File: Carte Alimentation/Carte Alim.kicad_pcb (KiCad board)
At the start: 2 copper layers, 102.9 x 70.5 mm, 58 parts, among them K1 CONN_3, P1 CONN_2, P10 CONN_2, P11 CONN_2, P12 CONN_2, P13 CONN_4, P2 CONN_2, P3 CONN_2, P4 CONN_5, P5 CONN_1, P6 CONN_1, P7 CONN_1, P8 CONN_1, P9 CONN_2, U100 7905_CORRIGE, U3 LM2903, U4 LM2903

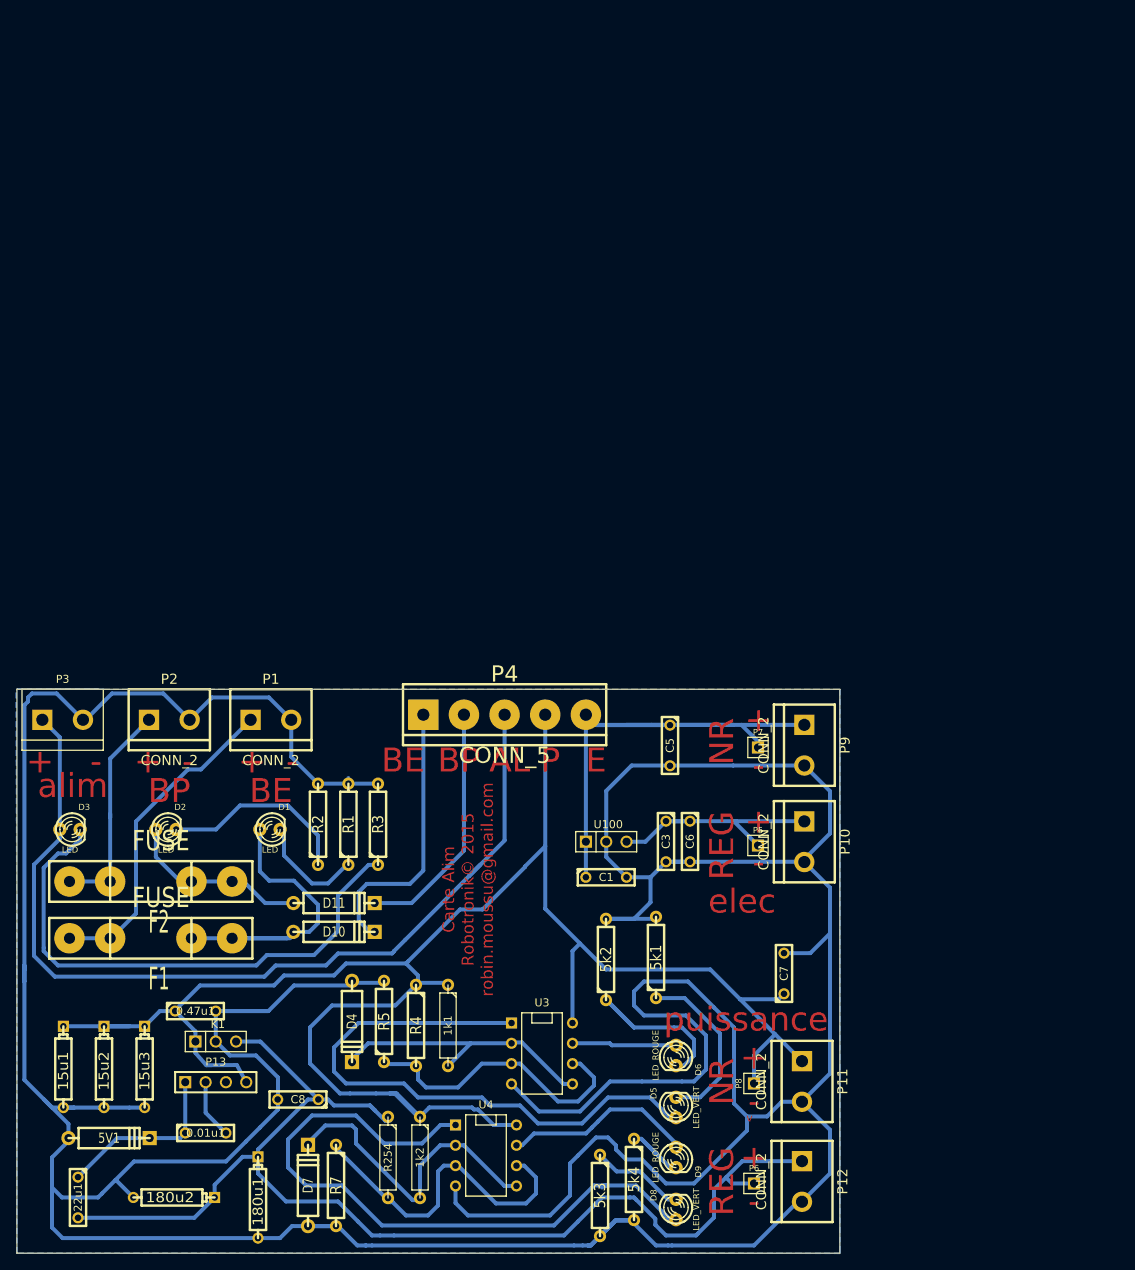
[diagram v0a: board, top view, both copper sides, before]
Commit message: some clean carte alim + export
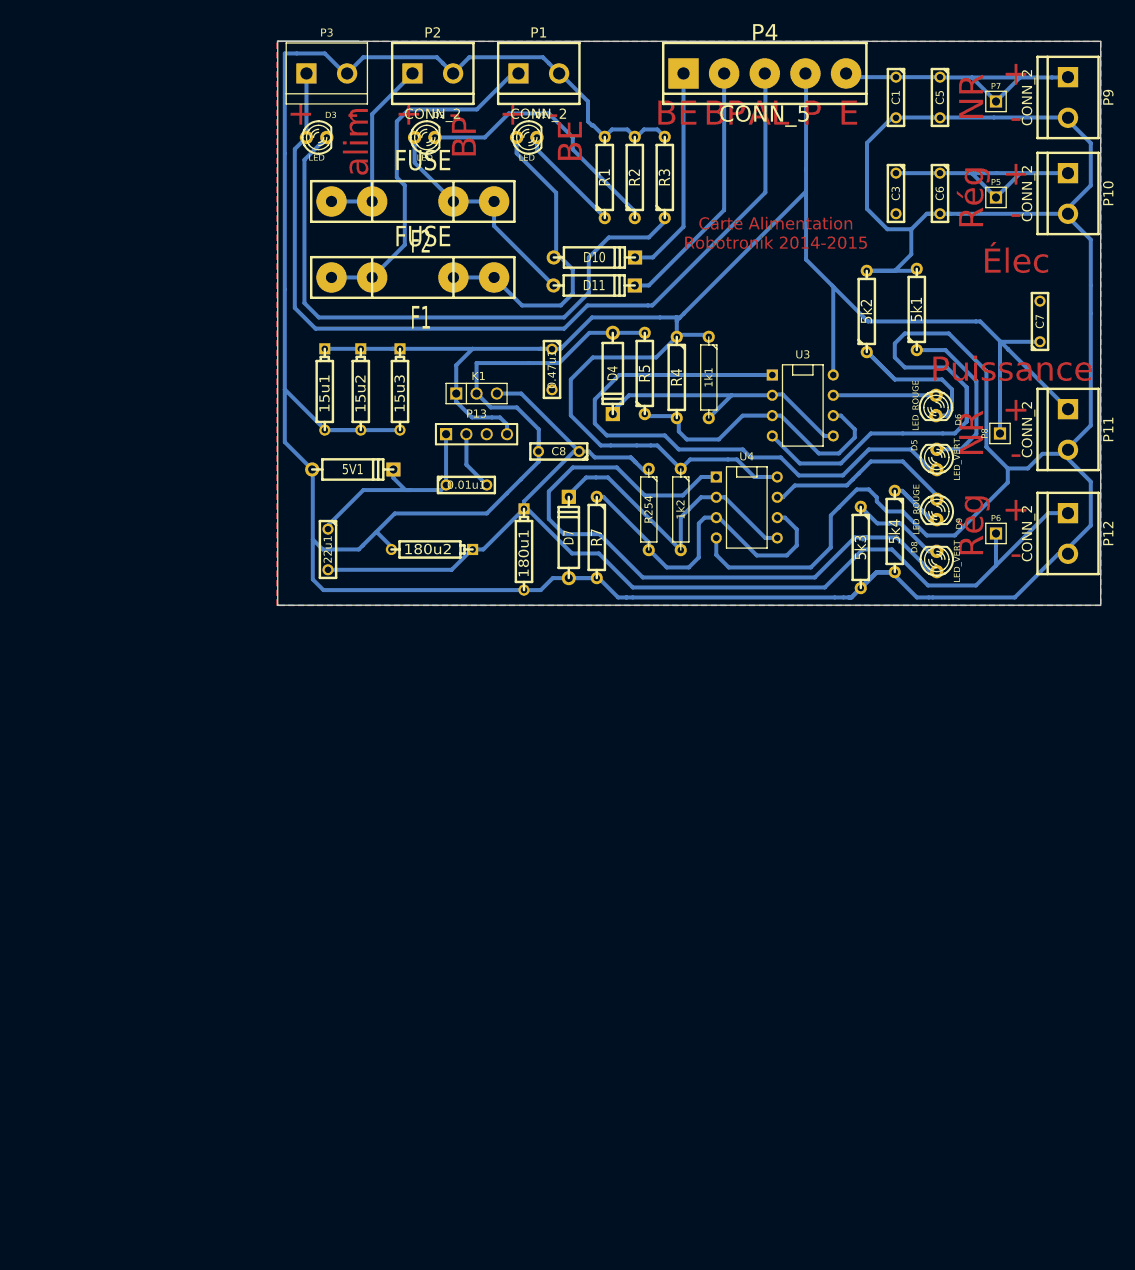
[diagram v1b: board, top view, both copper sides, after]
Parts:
- removed U100: 7905_CORRIGE, PIN_ARRAY_3X1
- moved C1 104.0 mm to (172.8, 83.5), turned to 270 degrees
- moved D2 92.4 mm to (113.8, 88.5)
- moved D1 92.3 mm to (126.6, 88.5)
- moved D3 91.8 mm to (100.3, 88.5)
- moved 0.47u1 91.8 mm to (129.8, 117.5), turned to 270 degrees
- moved F2 91.1 mm to (112.3, 96.5)
- moved 15u1 90.8 mm to (101.3, 120.0)
- moved 15u2 90.6 mm to (105.8, 120.0)
- moved 15u3 90.5 mm to (110.8, 120.0)
- moved D10 90.4 mm to (135.1, 103.5)
- moved R2 90.0 mm to (140.1, 93.5)
- moved 5V1 89.0 mm to (104.8, 130.0)
- moved F1 88.9 mm to (112.3, 106.0)
- moved R3 88.4 mm to (143.8, 93.5)
- moved P11 88.0 mm to (194.2, 125.0)
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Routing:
- net /alim_elec_non_regul: track 76.2 -> 35.9 mm
- net GND: track 628.2 -> 618.7 mm
- net Net-(D2-Pad2): track 24.2 -> 33.0 mm
- net Net-(D10-Pad2): track 34.8 -> 26.5 mm
- net Net-(D3-Pad2): track 68.1 -> 75.6 mm
- net Net-(D11-Pad1): track 23.0 -> 28.7 mm
- net Net-(0.01u1-Pad1): track 22.0 -> 27.5 mm
- net /alim_elec: track 34.9 -> 30.0 mm
- net Net-(F2-Pad1): track 27.7 -> 23.2 mm
- net Net-(D3-Pad1): track 116.4 -> 112.6 mm
- net Net-(F1-Pad1): track 41.1 -> 44.5 mm
- net /alim_puissance_regul: track 149.4 -> 146.1 mm
- net /alim_puissance_non_regul: track 237.9 -> 240.7 mm
- net Net-(D11-Pad2): track 30.9 -> 32.2 mm
- net Net-(1k2-Pad2): track 40.0 -> 38.9 mm
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- added copper zone on F.Cu, net GND
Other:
- board text added: "Carte Alimentation Robotronik 2014-2015"
- board text added: "Puissance"
- board text added: "Rég"
- board text added: "Élec"
- board text removed: "Carte Alim Robotronik© 2015 robin.moussu@gmail.com"
- board text removed: "REG"
- board text removed: "elec"
- board text removed: "puissance"
- board text removed: "v"
